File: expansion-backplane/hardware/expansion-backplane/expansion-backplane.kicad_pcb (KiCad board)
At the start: 2 copper layers, 100 x 51 mm, 15 parts, among them J1 Barrel_Jack, SW1 SW_SPDT

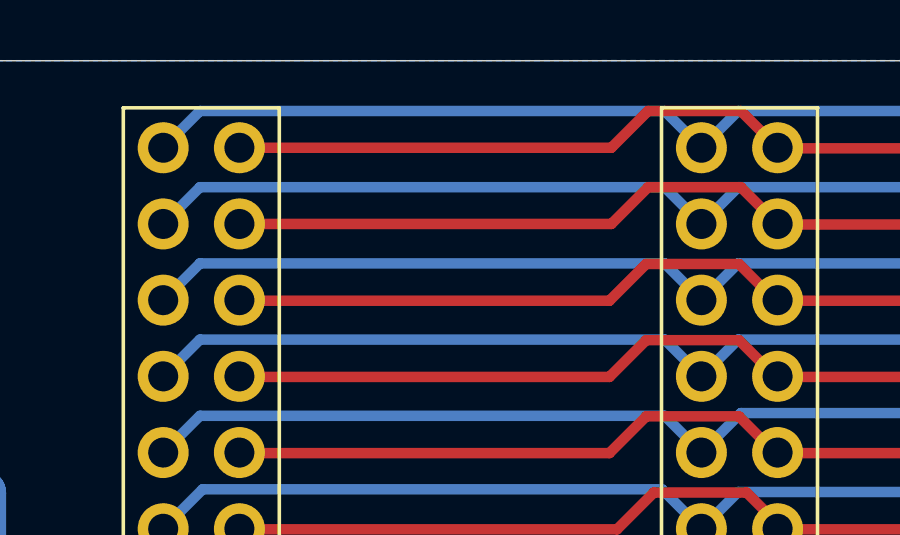
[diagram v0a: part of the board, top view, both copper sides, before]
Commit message: update speech pld file and more
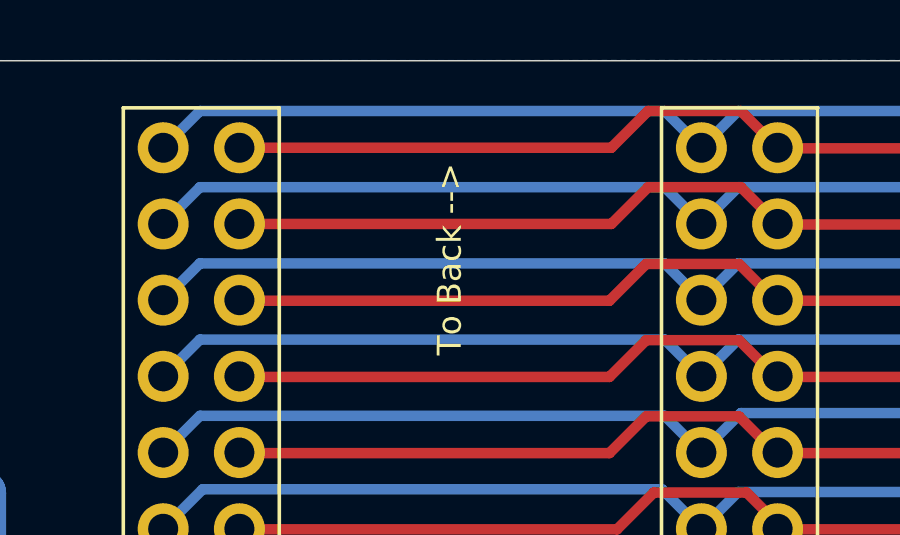
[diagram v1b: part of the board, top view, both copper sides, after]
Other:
- board text added: "To Back -->"
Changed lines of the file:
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@@
 			(outputformat 1)
 			(mirror no)
-			(drillshape 1)
+			(drillshape 0)
 			(scaleselection 1)
-			(outputdirectory "")
+			(outputdirectory "gerbers_v1")
 		)
 	)
@@
 		)
 	)
+	(gr_text "To Back -->"
+		(at 124.968 99.822 90)
+		(layer "F.SilkS")
+		(effects
+			(font
+				(size 0.8 0.8)
+				(thickness 0.1)
+			)
+			(justify left bottom)
+		)
+	)
